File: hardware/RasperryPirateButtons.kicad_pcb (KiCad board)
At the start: 2 copper layers, 65 x 56.5 mm, 19 parts, among them P1 CONN_01X04, P11 CONN_20X2, P2 CONN_01X04, P3 CONN_01X04, P4 CONN_01X04, Q1 MMBT3904, Q2 MMBT3904, Q3 MMBT3904, Q4 MMBT3904

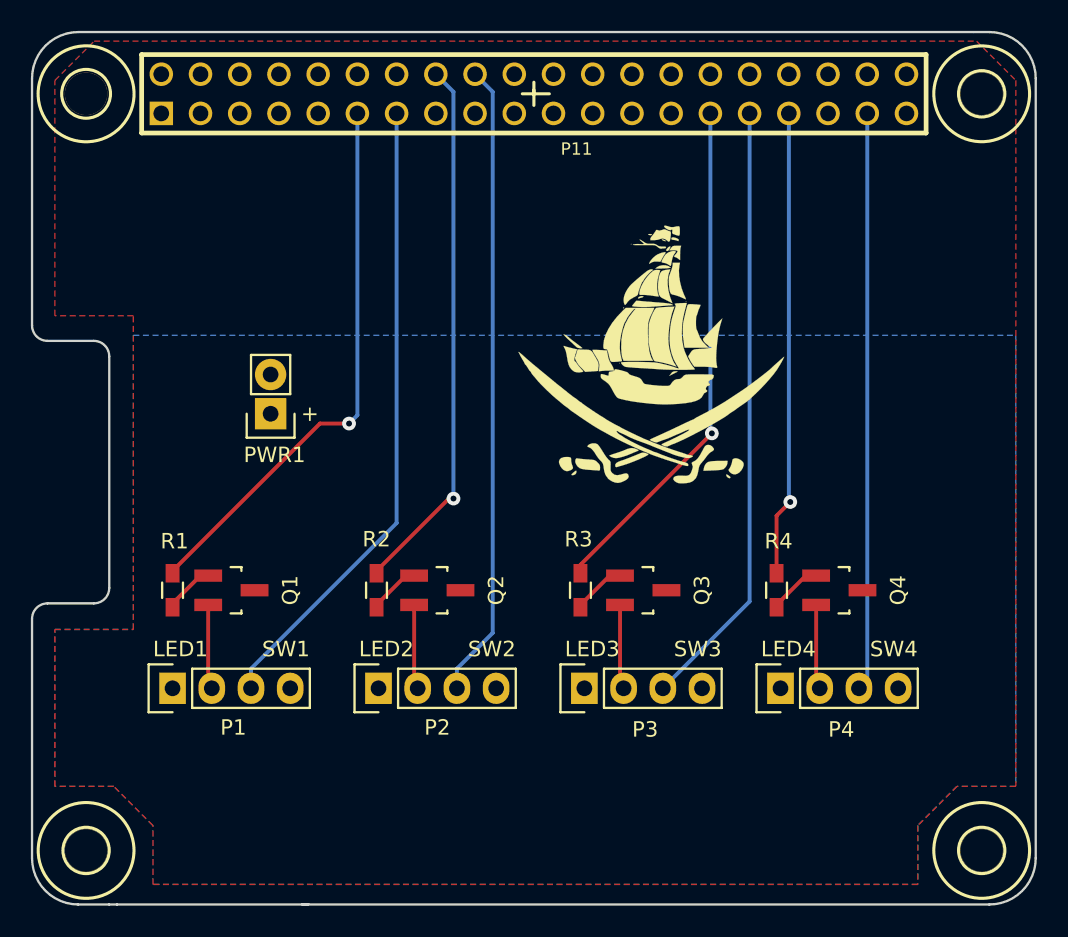
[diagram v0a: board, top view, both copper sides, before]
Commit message: Version 2 of pirate buttons
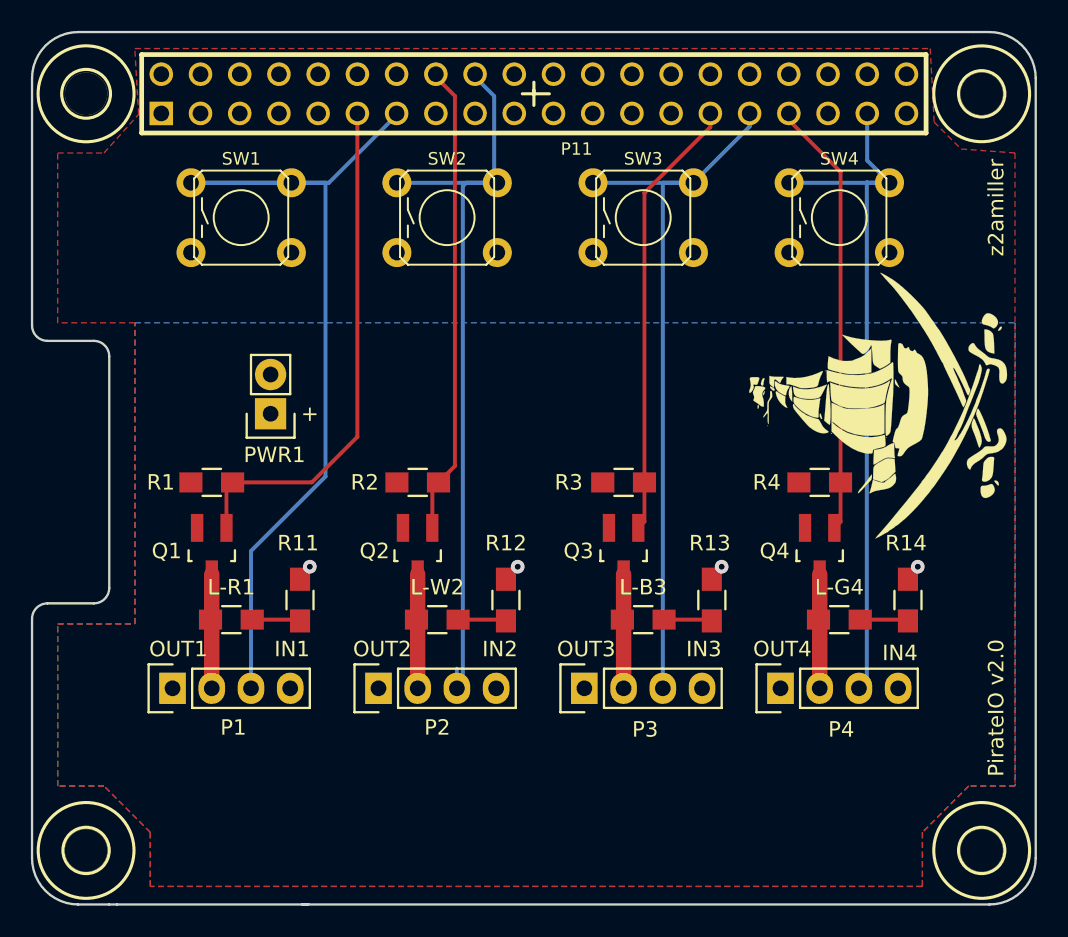
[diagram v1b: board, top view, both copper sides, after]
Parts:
- removed the G*** at (69.8, 41.9)
- added G***: LOGO, Kicad:pirateship, F.Cu at (83.8, 44.5)
- added L-B3: LED-B, Resistors_SMD:R_0805_HandSoldering, F.Cu at (68.6, 59.1)
- added L-G4: LED-G, Resistors_SMD:R_0805_HandSoldering, F.Cu at (81.3, 59.1)
- added L-R1: LED-R, Resistors_SMD:R_0805_HandSoldering, F.Cu at (41.9, 59.1)
- added L-W2: LED-W, Resistors_SMD:R_0805_HandSoldering, F.Cu at (55.2, 59.1)
- added R11: 560, Resistors_SMD:R_0805_HandSoldering, F.Cu at (46.4, 57.8)
- added R12: 560, Resistors_SMD:R_0805_HandSoldering, F.Cu at (59.7, 57.8)
- added R13: 560, Resistors_SMD:R_0805_HandSoldering, F.Cu at (73.0, 57.8)
- added R14: 560, Resistors_SMD:R_0805_HandSoldering, F.Cu at (85.7, 57.8)
- added SW1: BG SW, lib:AB2_PB_MOM_6MM_PTH_BLK, F.Cu at (42.5, 33.0)
- added SW2: BG SW, lib:AB2_PB_MOM_6MM_PTH_BLK, F.Cu at (55.9, 33.0)
- added SW3: BG SW, lib:AB2_PB_MOM_6MM_PTH_BLK, F.Cu at (68.6, 33.0)
- added SW4: BG SW, lib:AB2_PB_MOM_6MM_PTH_BLK, F.Cu at (81.3, 33.0)
- Q1, Q2, Q3, Q4: value MMBT3904 -> AO3400
- R1, R2, R3, R4: value 470 -> 100K; footprint Resistors_SMD:R_0603_HandSoldering -> Resistors_SMD:R_0805_HandSoldering
- moved R4 7.52 mm to (80.0, 50.2), turned to 180 degrees
- moved R3 7.52 mm to (67.3, 50.2), turned to 180 degrees
- moved R2 7.48 mm to (54.0, 50.2), turned to 180 degrees
- moved R1 7.43 mm to (40.6, 50.2), turned to 180 degrees
- moved Q1 2.84 mm to (40.6, 54.6), turned to 180 degrees
- moved Q2 2.84 mm to (54.0, 54.6), turned to 180 degrees
- moved Q3 2.84 mm to (67.3, 54.6), turned to 180 degrees
- moved Q4 2.84 mm to (80.0, 54.6), turned to 180 degrees
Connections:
- P1 pad 2: Net-(P1-Pad2) -> Net-(L-R1-Pad1)
- P2 pad 2: Net-(P2-Pad2) -> Net-(L-W2-Pad1)
- P3 pad 2: Net-(P3-Pad2) -> Net-(L-B3-Pad1)
- P4 pad 2: Net-(P4-Pad2) -> Net-(L-G4-Pad1)
- Q1 pad 1: Net-(Q1-Pad1) -> GPIO17
- Q1 pad 2: Net-(P1-Pad2) -> GND
- Q1 pad 3: GND -> Net-(L-R1-Pad1)
- Q2 pad 1: Net-(Q2-Pad1) -> GPIO23
- Q2 pad 2: Net-(P2-Pad2) -> GND
- Q2 pad 3: GND -> Net-(L-W2-Pad1)
- Q3 pad 1: Net-(Q3-Pad1) -> GPIO05
- Q3 pad 2: Net-(P3-Pad2) -> GND
- Q3 pad 3: GND -> Net-(L-B3-Pad1)
- Q4 pad 1: Net-(Q4-Pad1) -> GPIO13
- Q4 pad 2: Net-(P4-Pad2) -> GND
- Q4 pad 3: GND -> Net-(L-G4-Pad1)
- R1 pad 2: Net-(Q1-Pad1) -> GND
- R2 pad 2: Net-(Q2-Pad1) -> GND
- R3 pad 2: Net-(Q3-Pad1) -> GND
- R4 pad 2: Net-(Q4-Pad1) -> GND
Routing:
- net GPIO27: track 41.1 -> 60.0 mm
- net Net-(L-R1-Pad1): track 0.00 -> 10.8 mm
- net GPIO26: track 37.5 -> 46.8 mm
- net GPIO24: track 41.2 -> 50.0 mm
- net Net-(L-G4-Pad1): track 0.00 -> 7.72 mm
- net Net-(L-W2-Pad1): track 0.00 -> 7.72 mm
- net Net-(L-B3-Pad1): track 0.00 -> 7.72 mm
- net GPIO06: track 39.6 -> 47.2 mm
- net Net-(P4-Pad2): track 5.50 -> 0.00 mm
- net Net-(P2-Pad2): track 5.50 -> 0.00 mm
- net Net-(P1-Pad2): track 5.50 -> 0.00 mm
- net Net-(P3-Pad2): track 5.50 -> 0.00 mm
- net GPIO05: track 33.3 -> 28.8 mm, vias 1 -> 0
- net GPIO23: track 35.0 -> 30.5 mm, vias 1 -> 0
- net +12V: track 0.00 -> 4.34 mm, vias 0 -> 4
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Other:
- net class drain added: clearance 0.512, trace_width 1, via_dia 0.889, via_drill 0.381
- board text added: "IN1"
- board text added: "IN2"
- board text added: "IN3"
- board text added: "IN4"
- board text added: "OUT1"
- board text added: "OUT2"
- board text added: "OUT3"
- board text added: "OUT4"
- board text added: "PirateIO v2.0"
- board text added: "z2amiller"
- board text removed: "LED1"
- board text removed: "LED2"
- board text removed: "LED3"
- board text removed: "LED4"
- board text removed: "SW1"
- board text removed: "SW2"
- board text removed: "SW3"
- board text removed: "SW4"
